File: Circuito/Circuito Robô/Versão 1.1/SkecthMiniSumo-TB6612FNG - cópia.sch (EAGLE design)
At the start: 25 parts, among them IC1 LM317MB, U1 328P, Y1 16MHz

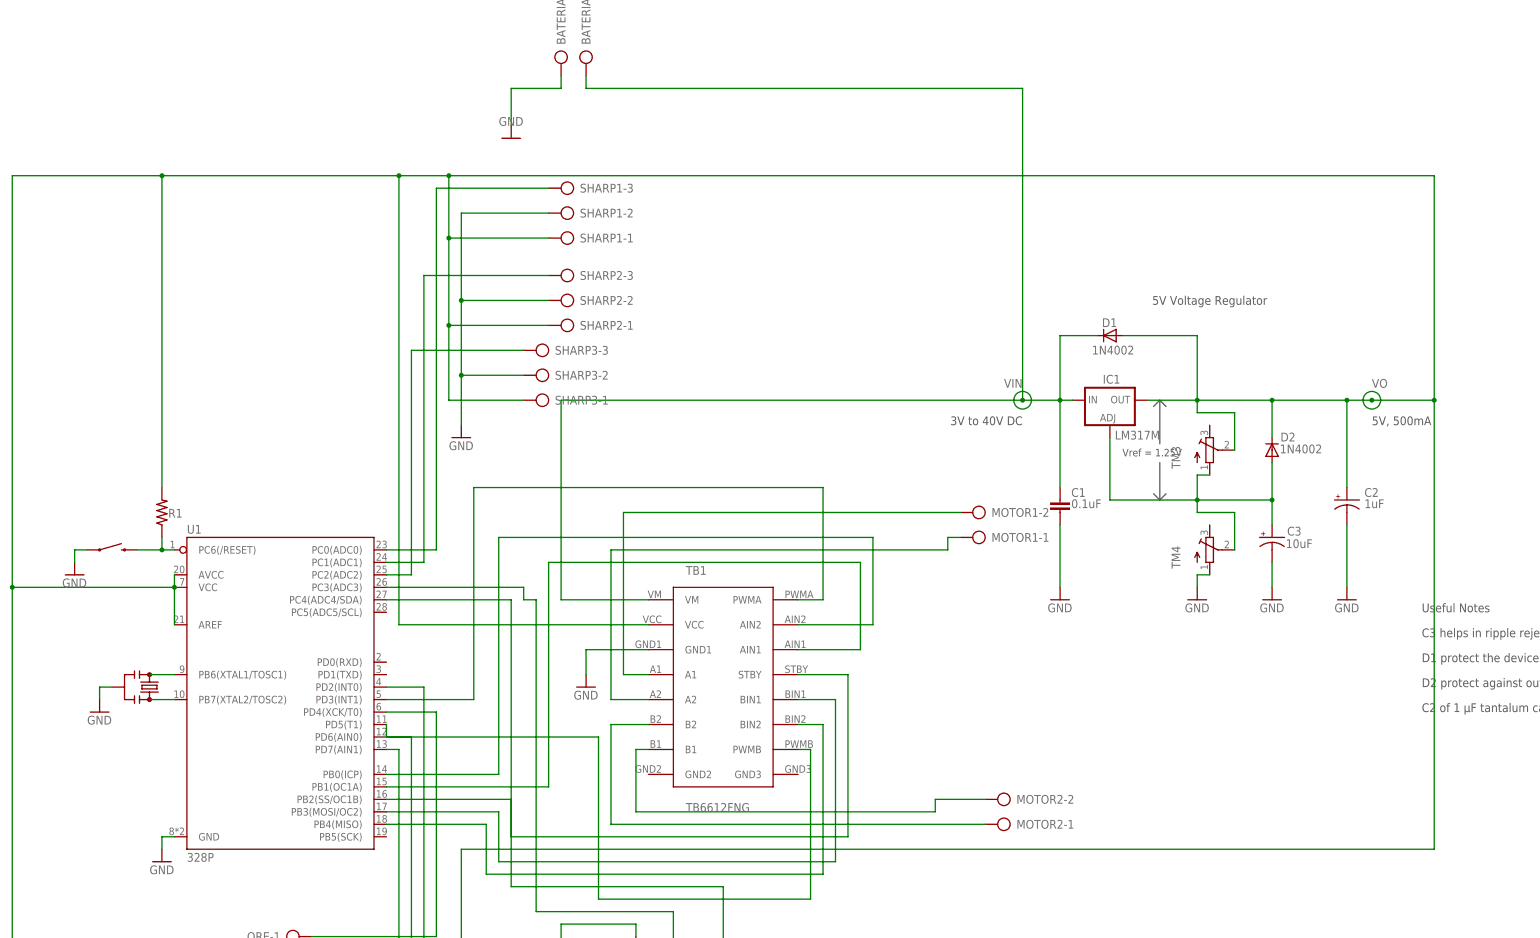
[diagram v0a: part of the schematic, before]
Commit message: Versão pós Luan
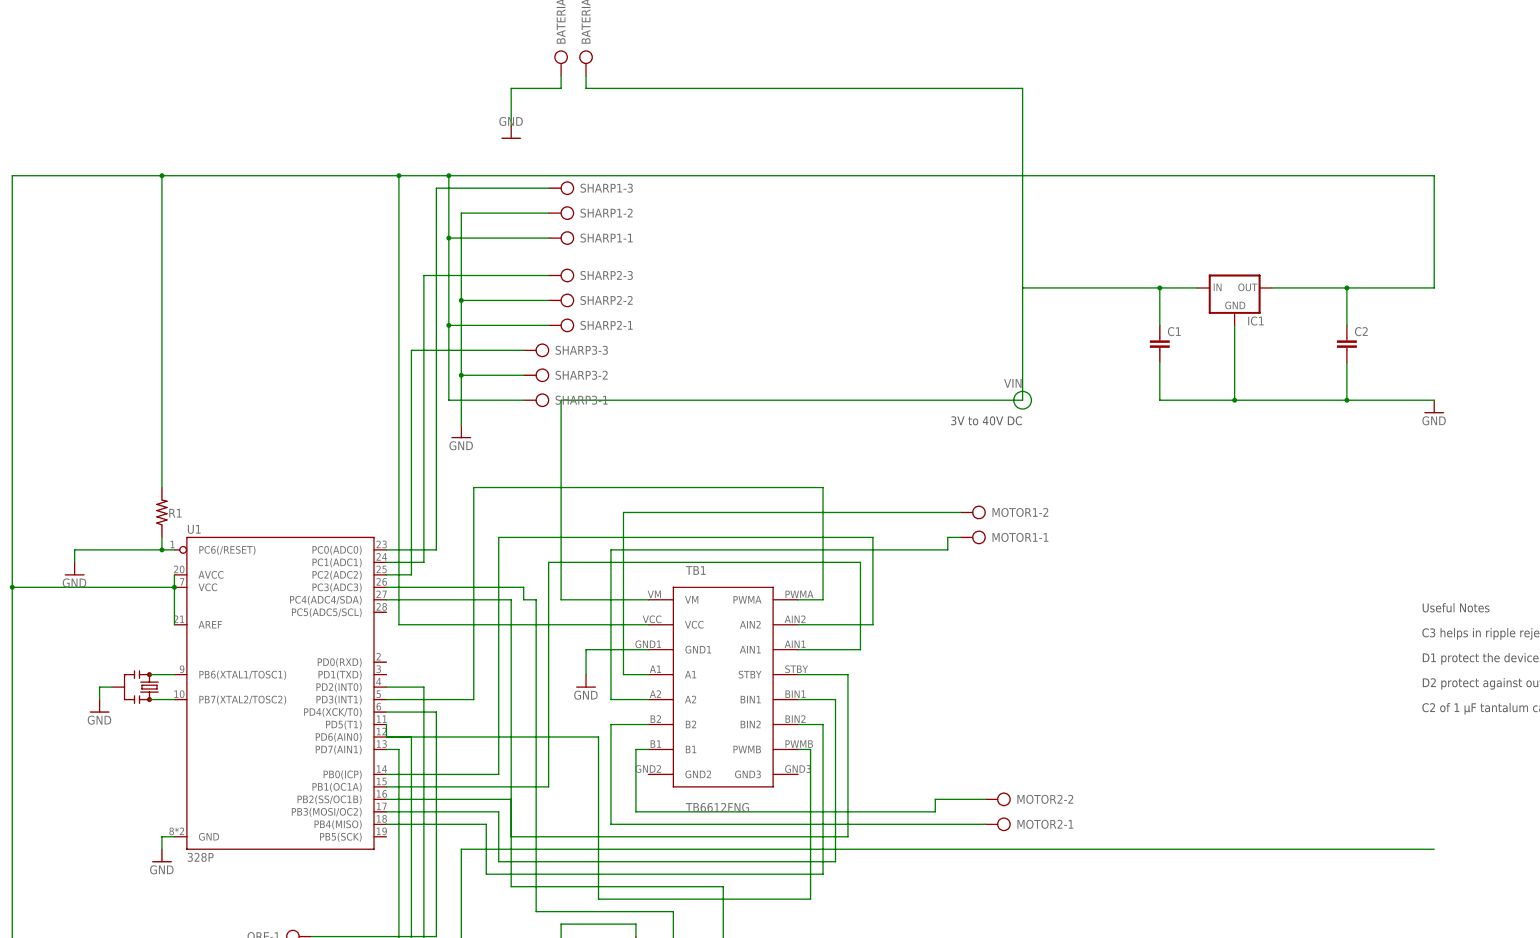
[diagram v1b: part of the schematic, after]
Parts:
- removed C3: 10uF, resistor:CPOL-US085CS-1AR
- removed D1, D2: 1N4002, diode:1N4004
- removed S1: MOMENTARY-SWITCH-SPST-SMD-6.2MM-TALL, SparkFun-Switches:MOMENTARY-SWITCH-SPST-SMD-6.2MM-TALL
- removed TM3, TM4: (no value), adafruit:TRIMPOT3386
- C1: value 0.1uF -> (none); device rcl:C-EU075-052X106 -> capacitor-wima:C5/3
- C2: value 1uF -> (none); device resistor:CPOL-US085CS-1AR -> capacitor-wima:C5/3
- IC1: value LM317MB -> (none); device v-reg:LM317MB -> v-reg:78LXX; PARTNUMBER LM317M -> (none)
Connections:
- removed net N$13: C3.+, D2.A, IC1.ADJ, TM3.A, TM4.S
- removed net N$3: R1.1, S1.2, U1.PC6(/RESET)
- new net N$32: QRE-3.KL, QRE2-3.KL, QRE3-3.KL, QRE4-3.KL
- net GND: now also C2.2, IC1.GND, R1.1, U1.PC6(/RESET); no longer C2.-, C3.-, S1.1, TM4.A
- net VIN: no longer D1.C
- net VO: now also C2.1; no longer C2.+, D1.A, D2.C, QRE-3.KL, QRE2-3.KL, QRE3-3.KL, QRE4-3.KL, TM3.S
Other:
- note removed: "5V Voltage Regulator"
- note removed: "5V, 500mA"
- note removed: "Vref = 1.25V"
- moved on the sheet: C1
